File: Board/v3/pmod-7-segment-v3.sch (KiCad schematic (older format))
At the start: 17 parts, among them J1 PMOD

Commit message: v3: initial schematic
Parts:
- removed J1: PMOD, Digilent:PMOD-DUAL-MALE, symbol pmod-7-segment-v2-rescue:PMOD-pmod-7-segment-v2-rescue
- removed LED1, LED2, LED3, LED4, LED5, LED6, LED7, LED8: SA39-11, Kingbright:SA39-11, symbol pmod-7-segment-v2-rescue:SA39-11-pmod-7-segment-v2-rescue
- removed R1, R2, R3, R4, R5, R6, R7, R8: R, Resistors_SMD:R_0603, symbol pmod-7-segment-v2-rescue:R-pmod-7-segment-v2-rescue
- added LED1, LED2, LED3, LED4, LED5, LED6, LED7, LED8: SUNLIGHT_SMD_7SEG_SLS0561, symbol tom-opto:SUNLIGHT_SMD_7SEG_SLS0561
- added R?: 47R, symbol tom-passives:R
- added R? (x7): R, symbol tom-passives:R
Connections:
- net labels added: D1_R, D2_R, D3_R, D4_R, D5_R, D6_R, D7_R, D8_R
- net labels removed: GND, S0, S1, S2, S3, S4, S5, S6, S7
- wire segments 90 -> 168
- no-connect marks 11 -> 8

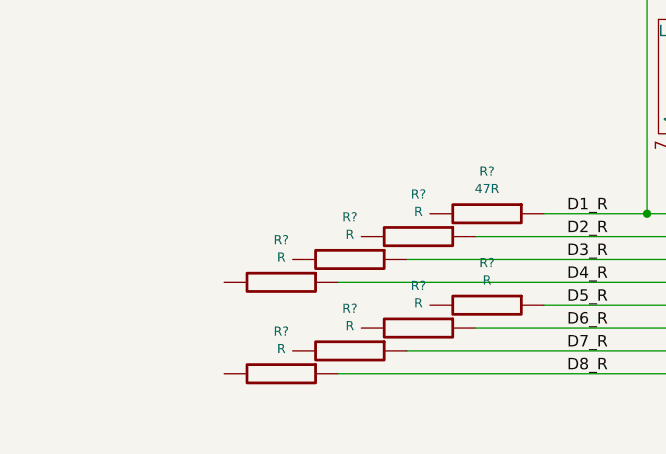
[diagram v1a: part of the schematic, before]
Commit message: v3: v3.0 as sent to jlcpcb
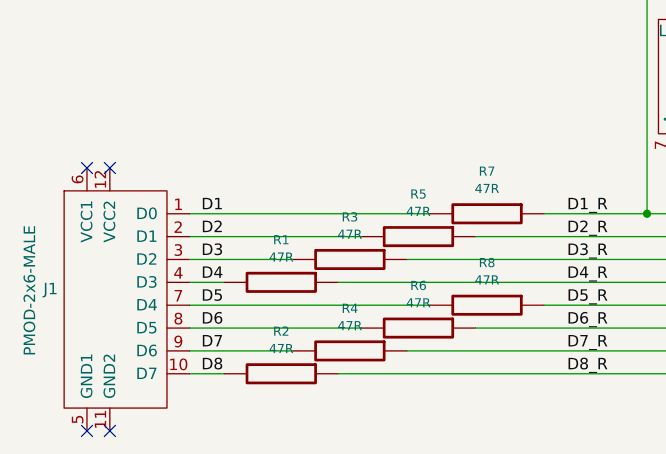
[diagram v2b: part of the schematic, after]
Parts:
- removed R? (x6): R, symbol tom-passives:R
- added J1: PMOD-2x6-MALE, tom-connectors:PMOD_2X6_PTH_RA_PLUG, symbol tom-connectors:PMOD-2x6-MALE
- added R1, R2, R3, R4, R6, R8: 47R, tom-passives:R_0603_1608Metric, symbol tom-passives:R
- LED1, LED2, LED3, LED4, LED5, LED6, LED7, LED8: footprint (none) -> tom-opto:SUNLIGHT_SMD_7SEG_SLS0561
- R5: renamed from R?; value R -> 47R; footprint (none) -> tom-passives:R_0603_1608Metric
- R7: renamed from R?; footprint (none) -> tom-passives:R_0603_1608Metric
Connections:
- net labels added: D1, D2, D3, D4, D5, D6, D7, D8
- wire segments 168 -> 176
- no-connect marks 8 -> 12
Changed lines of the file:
@@
 EESchema Schematic File Version 4
+LIBS:pmod-7-segment-v3-cache
 EELAYER 30 0
 EELAYER END
@@
 F 0 "LED1" H 3650 3250 50  0000 L CNN
 F 1 "SUNLIGHT_SMD_7SEG_SLS0561" V 3450 3900 50  0000 L CNN
-F 2 "" H 4050 3050 50  0001 C CNN
+F 2 "tom-opto:SUNLIGHT_SMD_7SEG_SLS0561" H 4050 3050 50  0001 C CNN
 F 3 "" H 4050 3050 50  0001 C CNN
 	1    4050 3050
@@
 F 0 "LED2" H 4550 3250 50  0000 L CNN
 F 1 "SUNLIGHT_SMD_7SEG_SLS0561" V 4350 3900 50  0000 L CNN
-F 2 "" H 4950 3050 50  0001 C CNN
+F 2 "tom-opto:SUNLIGHT_SMD_7SEG_SLS0561" H 4950 3050 50  0001 C CNN
 F 3 "" H 4950 3050 50  0001 C CNN
 	1    4950 3050
@@
 F 0 "LED3" H 5450 3250 50  0000 L CNN
 F 1 "SUNLIGHT_SMD_7SEG_SLS0561" V 5250 3900 50  0000 L CNN
-F 2 "" H 5850 3050 50  0001 C CNN
+F 2 "tom-opto:SUNLIGHT_SMD_7SEG_SLS0561" H 5850 3050 50  0001 C CNN
 F 3 "" H 5850 3050 50  0001 C CNN
 	1    5850 3050
@@
 F 0 "LED4" H 6350 3250 50  0000 L CNN
 F 1 "SUNLIGHT_SMD_7SEG_SLS0561" V 6150 3900 50  0000 L CNN
-F 2 "" H 6750 3050 50  0001 C CNN
+F 2 "tom-opto:SUNLIGHT_SMD_7SEG_SLS0561" H 6750 3050 50  0001 C CNN
 F 3 "" H 6750 3050 50  0001 C CNN
 	1    6750 3050
@@
 F 0 "LED5" H 7250 3250 50  0000 L CNN
 F 1 "SUNLIGHT_SMD_7SEG_SLS0561" V 7050 3900 50  0000 L CNN
-F 2 "" H 7650 3050 50  0001 C CNN
+F 2 "tom-opto:SUNLIGHT_SMD_7SEG_SLS0561" H 7650 3050 50  0001 C CNN
 F 3 "" H 7650 3050 50  0001 C CNN
 	1    7650 3050
@@
 F 0 "LED6" H 8150 3250 50  0000 L CNN
 F 1 "SUNLIGHT_SMD_7SEG_SLS0561" V 7950 3900 50  0000 L CNN
-F 2 "" H 8550 3050 50  0001 C CNN
+F 2 "tom-opto:SUNLIGHT_SMD_7SEG_SLS0561" H 8550 3050 50  0001 C CNN
 F 3 "" H 8550 3050 50  0001 C CNN
 	1    8550 3050
@@
 F 0 "LED7" H 9050 3250 50  0000 L CNN
 F 1 "SUNLIGHT_SMD_7SEG_SLS0561" V 8850 3900 50  0000 L CNN
-F 2 "" H 9450 3050 50  0001 C CNN
+F 2 "tom-opto:SUNLIGHT_SMD_7SEG_SLS0561" H 9450 3050 50  0001 C CNN
 F 3 "" H 9450 3050 50  0001 C CNN
 	1    9450 3050
@@
 F 0 "LED8" H 9950 3250 50  0000 L CNN
 F 1 "SUNLIGHT_SMD_7SEG_SLS0561" V 9750 3900 50  0000 L CNN
-F 2 "" H 10350 3050 50  0001 C CNN
+F 2 "tom-opto:SUNLIGHT_SMD_7SEG_SLS0561" H 10350 3050 50  0001 C CNN
 F 3 "" H 10350 3050 50  0001 C CNN
 	1    10350 3050
@@
 D8_R
 $Comp
-L tom-passives:R R?
+L tom-passives:R R7
 U 1 1 5DF37CE5
 P 2900 3650
-F 0 "R?" V 2715 3650 40  0000 C CNN
+F 0 "R7" V 2715 3650 40  0000 C CNN
 F 1 "47R" V 2791 3650 40  0000 C CNN
-F 2 "" V 2830 3650 30  0000 C CNN
+F 2 "tom-passives:R_0603_1608Metric" V 2830 3650 30  0001 C CNN
 F 3 "" H 2900 3650 30  0000 C CNN
 	1    2900 3650
@@
 $EndComp
 $Comp
-L tom-passives:R R?
+L tom-passives:R R5
 U 1 1 5DF38E83
 P 2600 3750
-F 0 "R?" V 2415 3750 40  0000 C CNN
-F 1 "R" V 2491 3750 40  0000 C CNN
-F 2 "" V 2530 3750 30  0000 C CNN
+F 0 "R5" V 2415 3750 40  0000 C CNN
+F 1 "47R" V 2491 3750 40  0000 C CNN
+F 2 "tom-passives:R_0603_1608Metric" V 2530 3750 30  0001 C CNN
 F 3 "" H 2600 3750 30  0000 C CNN
 	1    2600 3750
 	0    1    1    0
 $EndComp
-$Comp
-L tom-passives:R R?
-U 1 1 5DF3950A
+Wire Wire Line
+	2850 3750 3700 3750
+Wire Wire Line
+	2550 3850 3800 3850
+Wire Wire Line
+	2250 3950 3900 3950
+Wire Wire Line
+	2850 4150 4100 4150
+Wire Wire Line
+	2550 4250 4200 4250
+Wire Wire Line
+	2250 4350 4300 4350
+$Comp
+L tom-passives:R R3
+U 1 1 5DD7BB2A
 P 2300 3850
-F 0 "R?" V 2115 3850 40  0000 C CNN
-F 1 "R" V 2191 3850 40  0000 C CNN
-F 2 "" V 2230 3850 30  0000 C CNN
+F 0 "R3" V 2115 3850 40  0000 C CNN
+F 1 "47R" V 2191 3850 40  0000 C CNN
+F 2 "tom-passives:R_0603_1608Metric" V 2230 3850 30  0001 C CNN
 F 3 "" H 2300 3850 30  0000 C CNN
 	1    2300 3850
@@
 $EndComp
 $Comp
-L tom-passives:R R?
-U 1 1 5DF39E33
+L tom-passives:R R1
+U 1 1 5DD7BD69
 P 2000 3950
-F 0 "R?" V 1815 3950 40  0000 C CNN
-F 1 "R" V 1891 3950 40  0000 C CNN
-F 2 "" V 1930 3950 30  0000 C CNN
+F 0 "R1" V 1815 3950 40  0000 C CNN
+F 1 "47R" V 1891 3950 40  0000 C CNN
+F 2 "tom-passives:R_0603_1608Metric" V 1930 3950 30  0001 C CNN
 F 3 "" H 2000 3950 30  0000 C CNN
 	1    2000 3950
@@
 $EndComp
 $Comp
-L tom-passives:R R?
-U 1 1 5DF3AB6C
+L tom-passives:R R8
+U 1 1 5DD7BFCD
 P 2900 4050
-F 0 "R?" V 2715 4050 40  0000 C CNN
-F 1 "R" V 2791 4050 40  0000 C CNN
-F 2 "" V 2830 4050 30  0000 C CNN
+F 0 "R8" V 2715 4050 40  0000 C CNN
+F 1 "47R" V 2791 4050 40  0000 C CNN
+F 2 "tom-passives:R_0603_1608Metric" V 2830 4050 30  0001 C CNN
 F 3 "" H 2900 4050 30  0000 C CNN
 	1    2900 4050
@@
 $EndComp
 $Comp
-L tom-passives:R R?
-U 1 1 5DF3AB76
+L tom-passives:R R6
+U 1 1 5DD7C2AC
 P 2600 4150
-F 0 "R?" V 2415 4150 40  0000 C CNN
-F 1 "R" V 2491 4150 40  0000 C CNN
-F 2 "" V 2530 4150 30  0000 C CNN
+F 0 "R6" V 2415 4150 40  0000 C CNN
+F 1 "47R" V 2491 4150 40  0000 C CNN
+F 2 "tom-passives:R_0603_1608Metric" V 2530 4150 30  0001 C CNN
 F 3 "" H 2600 4150 30  0000 C CNN
 	1    2600 4150
@@
 $EndComp
 $Comp
-L tom-passives:R R?
-U 1 1 5DF3AB80
+L tom-passives:R R4
+U 1 1 5DD7C4C0
 P 2300 4250
-F 0 "R?" V 2115 4250 40  0000 C CNN
-F 1 "R" V 2191 4250 40  0000 C CNN
-F 2 "" V 2230 4250 30  0000 C CNN
+F 0 "R4" V 2115 4250 40  0000 C CNN
+F 1 "47R" V 2191 4250 40  0000 C CNN
+F 2 "tom-passives:R_0603_1608Metric" V 2230 4250 30  0001 C CNN
 F 3 "" H 2300 4250 30  0000 C CNN
 	1    2300 4250
@@
 $EndComp
 $Comp
-L tom-passives:R R?
-U 1 1 5DF3AB8A
+L tom-passives:R R2
+U 1 1 5DD7C7AC
 P 2000 4350
-F 0 "R?" V 1815 4350 40  0000 C CNN
-F 1 "R" V 1891 4350 40  0000 C CNN
-F 2 "" V 1930 4350 30  0000 C CNN
+F 0 "R2" V 1815 4350 40  0000 C CNN
+F 1 "47R" V 1891 4350 40  0000 C CNN
+F 2 "tom-passives:R_0603_1608Metric" V 1930 4350 30  0001 C CNN
 F 3 "" H 2000 4350 30  0000 C CNN
 	1    2000 4350
 	0    1    1    0
 $EndComp
-Wire Wire Line
-	2850 3750 3700 3750
-Wire Wire Line
-	2550 3850 3800 3850
-Wire Wire Line
-	2250 3950 3900 3950
-Wire Wire Line
-	2850 4150 4100 4150
-Wire Wire Line
-	2550 4250 4200 4250
-Wire Wire Line
-	2250 4350 4300 4350
+$Comp
+L tom-connectors:PMOD-2x6-MALE J1
+U 1 1 5DD7CA6E
+P 1350 3900
+F 0 "J1" H 1023 3821 50  0000 R CNN
+F 1 "PMOD-2x6-MALE" V 900 4100 50  0000 R CNN
+F 2 "tom-connectors:PMOD_2X6_PTH_RA_PLUG" H 1350 3900 50  0001 C CNN
+F 3 "" H 1350 3900 50  0001 C CNN
+	1    1350 3900
+	1    0    0    -1
+$EndComp
+NoConn ~ 1250 3450
+NoConn ~ 1150 3450
+NoConn ~ 1250 4600
+NoConn ~ 1150 4600
+Wire Wire Line
+	1600 3650 2650 3650
+Wire Wire Line
+	2350 3750 1600 3750
+Wire Wire Line
+	1600 3850 2050 3850
+Wire Wire Line
+	1750 3950 1600 3950
+Wire Wire Line
+	1600 4050 2650 4050
+Wire Wire Line
+	2350 4150 1600 4150
+Wire Wire Line
+	1600 4250 2050 4250
+Wire Wire Line
+	1750 4350 1600 4350
+Text Label 1650 3650 0    50   ~ 0
+D1
+Text Label 1650 3750 0    50   ~ 0
+D2
+Text Label 1650 3850 0    50   ~ 0
+D3
+Text Label 1650 3950 0    50   ~ 0
+D4
+Text Label 1650 4050 0    50   ~ 0
+D5
+Text Label 1650 4150 0    50   ~ 0
+D6
+Text Label 1650 4250 0    50   ~ 0
+D7
+Text Label 1650 4350 0    50   ~ 0
+D8
 $EndSCHEMATC
